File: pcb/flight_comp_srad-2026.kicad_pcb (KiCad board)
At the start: 4 copper layers, 70 x 40 mm, 69 parts, among them J1 503398-1892, J2 Connector_3, J3 USB_B_Micro, J5 Vin_Bat, U1 IIM-20670, U2 NCP1117-3.3_SOT223, U3 RP2040, U4 ADXL375BCCZ-RL7, U5 MAX-M10M-00B, U6 W25Q128JVS, U7 XBP9B-DMSTB002, Y1 ABM8-272-T3

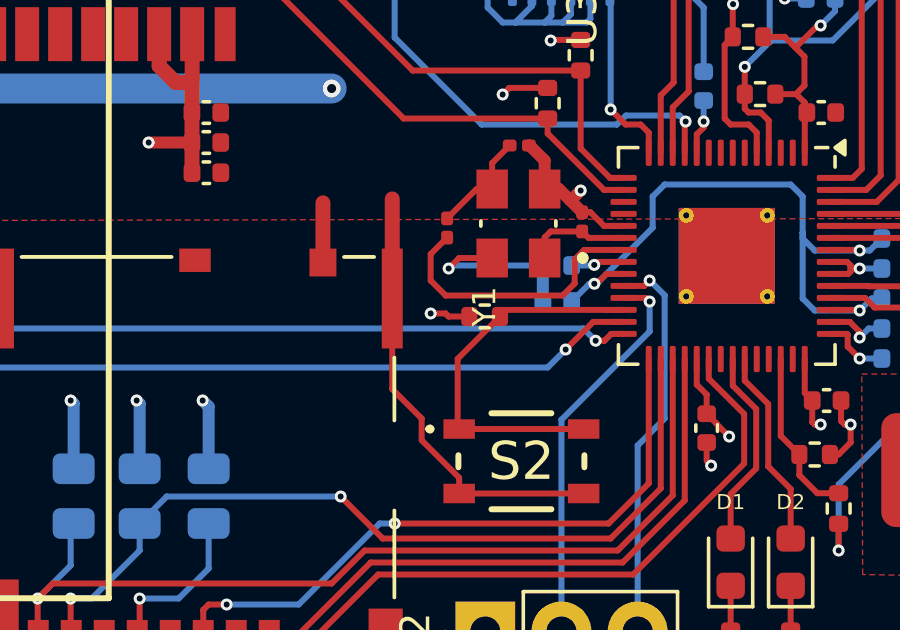
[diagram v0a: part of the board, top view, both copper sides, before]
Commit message: agregue coments
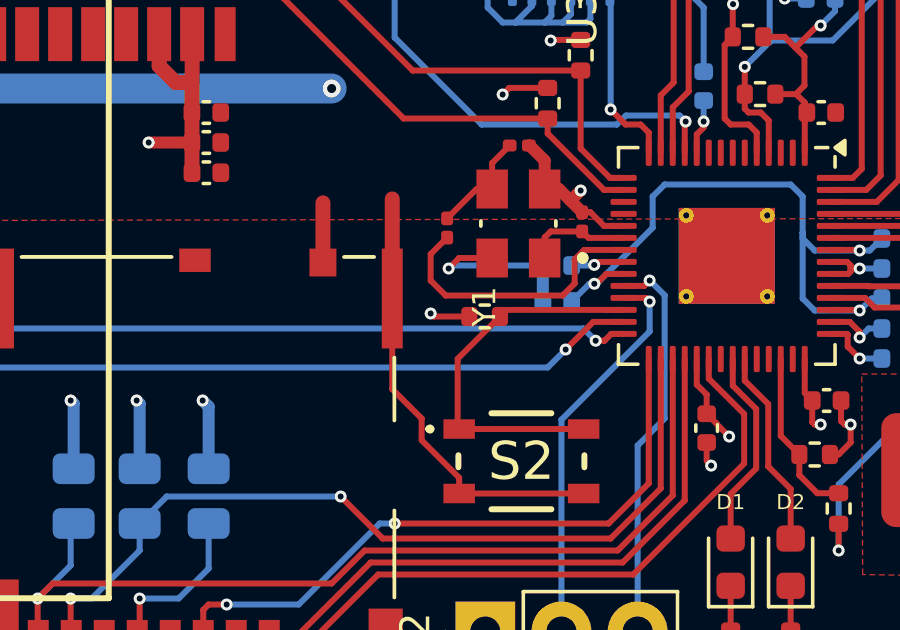
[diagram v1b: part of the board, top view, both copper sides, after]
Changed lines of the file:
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@@
 	)
 	(segment
-		(start 190.699 88.099)
-		(end 190.8 88.2)
+		(start 190.301 88.2)
+		(end 191.49 88.2)
 		(width 0.2)
 		(layer "F.Cu")
@@
 		(start 212.835 68.05)
 		(end 212.835 67.16)
-		(width 0.2)
-		(layer "F.Cu")
-		(net 47)
-	)
-	(segment
-		(start 190.8 88.2)
-		(end 191.49 88.2)
 		(width 0.2)
 		(layer "F.Cu")
@@
 	)
 	(segment
-		(start 190.2 88.099)
-		(end 190.699 88.099)
-		(width 0.2)
-		(layer "F.Cu")
-		(net 47)
-	)
-	(segment
 		(start 204.5 88.708521)
 		(end 204.5 88.9)
 		(width 0.2)
 		(layer "F.Cu")
+		(net 47)
+	)
+	(segment
+		(start 190.2 88.099)
+		(end 190.301 88.2)
+		(width 0.2)
+		(layer "F.Cu")
